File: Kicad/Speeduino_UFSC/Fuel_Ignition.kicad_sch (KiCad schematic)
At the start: 17 parts, among them Q1 Q_NMOS_GDS, U1 TC4424A

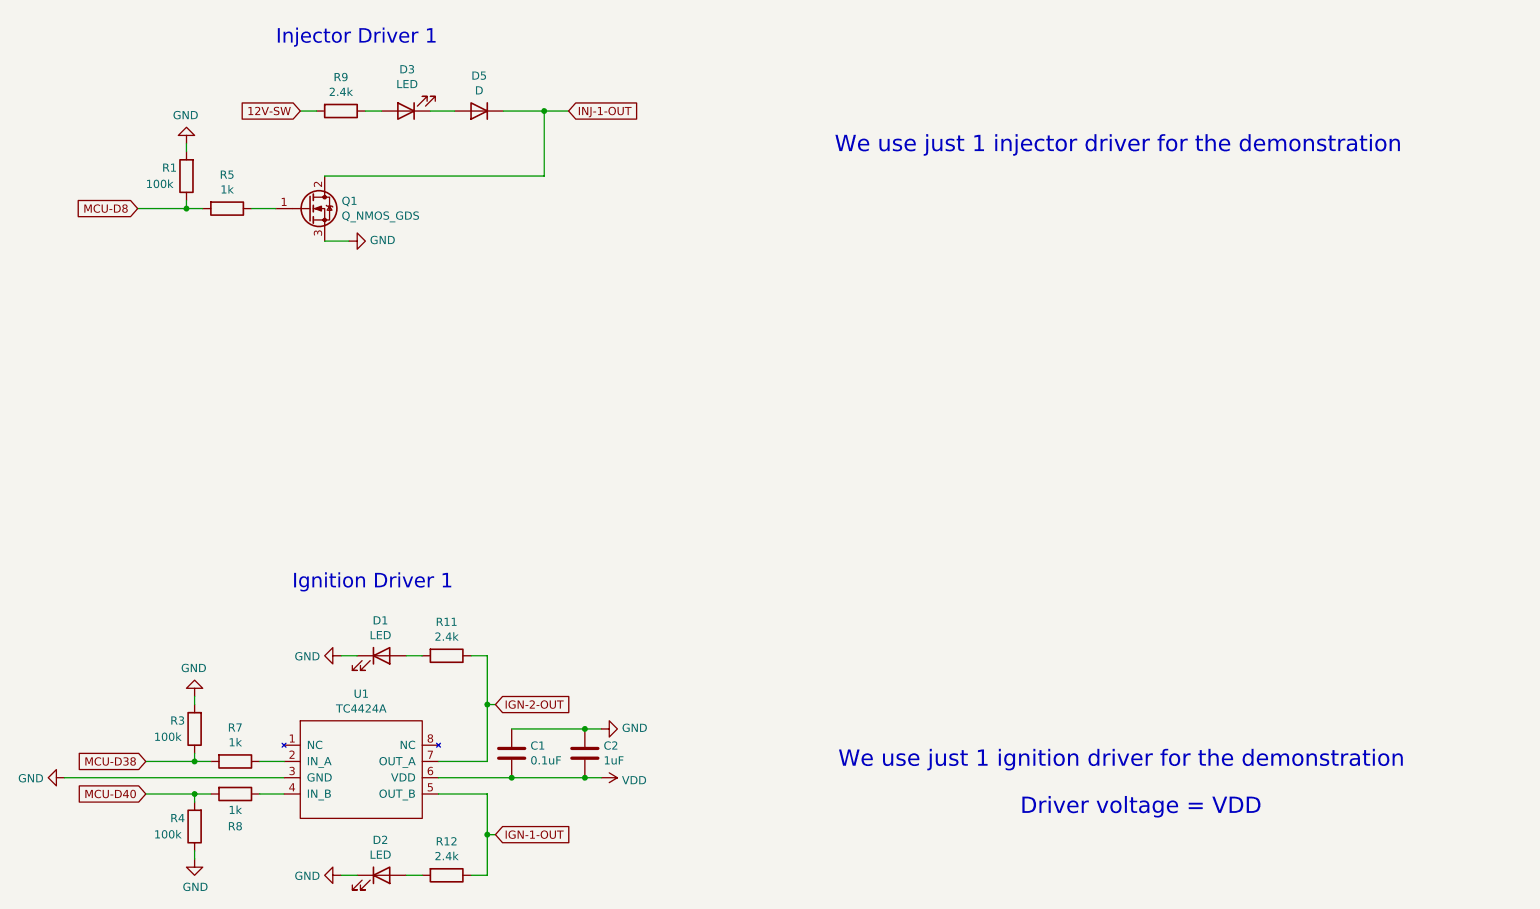
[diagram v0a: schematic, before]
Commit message: Update Kicad
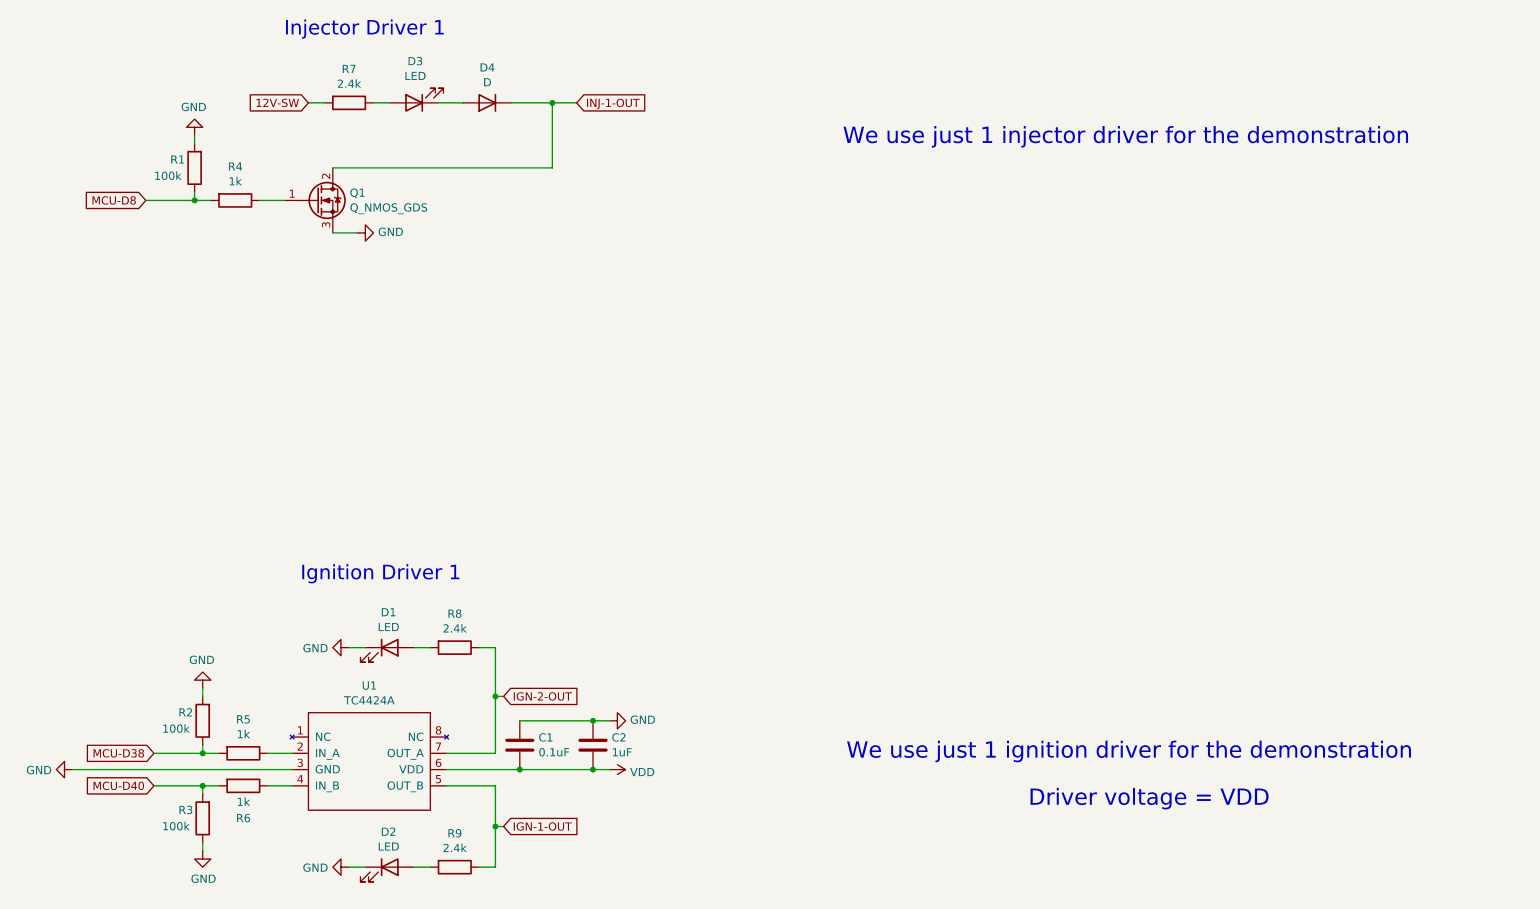
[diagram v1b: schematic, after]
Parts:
- removed D5: D, Diode_THT:D_DO-35_SOD27_P7.62mm_Horizontal, symbol Device:D
- removed R11, R12: 2.4k, Resistor_THT:R_Axial_DIN0204_L3.6mm_D1.6mm_P5.08mm_Horizontal, symbol Device:R
- added D4: D, Diode_THT:D_DO-35_SOD27_P7.62mm_Horizontal, symbol Device:D
- added R2: 100k, Resistor_THT:R_Axial_DIN0204_L3.6mm_D1.6mm_P5.08mm_Horizontal, symbol Device:R
- added R6: 1k, Resistor_THT:R_Axial_DIN0204_L3.6mm_D1.6mm_P5.08mm_Horizontal, symbol Device:R
- R4: value 100k -> 1k; Digikey Part Number BC3240CT-ND -> BC1.00KXCT-ND; Manufacturer_Part_Number MBA02040C1003FCT00 -> MBA02040C1001FRP00; URL https://www.digikey.com.au/product-detail/en/vishay-beyschl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 -> (none)
- R7, R8: value 1k -> 2.4k; Digikey Part Number BC1.00KXCT-ND -> BC3483CT-ND; Manufacturer_Part_Number MBA02040C1001FRP00 -> MBA02040C2401FC100; URL (none) -> https://www.digikey.com.au/product-detail/en/vishay-beyschl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
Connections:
- net 12V-SW: now also R7.2; no longer R9.2
- net GND: now also R3.1, R2.2; no longer R3.2, R4.1
- net IGN-1-OUT: now also R9.1
- net IGN-2-OUT: now also R8.1
- net INJ-1-OUT: now also D4.1 (K)
- net MCU-D38: now also R5.2, R2.1; no longer R3.1, R7.2
- net MCU-D40: now also R3.2, R6.2; no longer R4.2, R8.2
- net MCU-D8: now also R4.2; no longer R5.2
- net at R7.1: now also D3.2 (A); no longer U1.2 (IN_A)
- net at U1.4 (IN_B): now also R6.1; no longer R8.1
- net at D1.2 (A): now also R8.2
- net at D3.1 (K): now also D4.2 (A)
- net at D2.2 (A): now also R9.2
- net at Q1.1 (G): now also R4.1; no longer R5.1
- new net: R5.1, U1.2 (IN_A)
